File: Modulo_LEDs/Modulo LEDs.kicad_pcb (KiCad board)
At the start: 2 copper layers, 33 x 61.6 mm, 18 parts, among them J1 Conn_01x09_Female, J2 Conn_01x09_Male

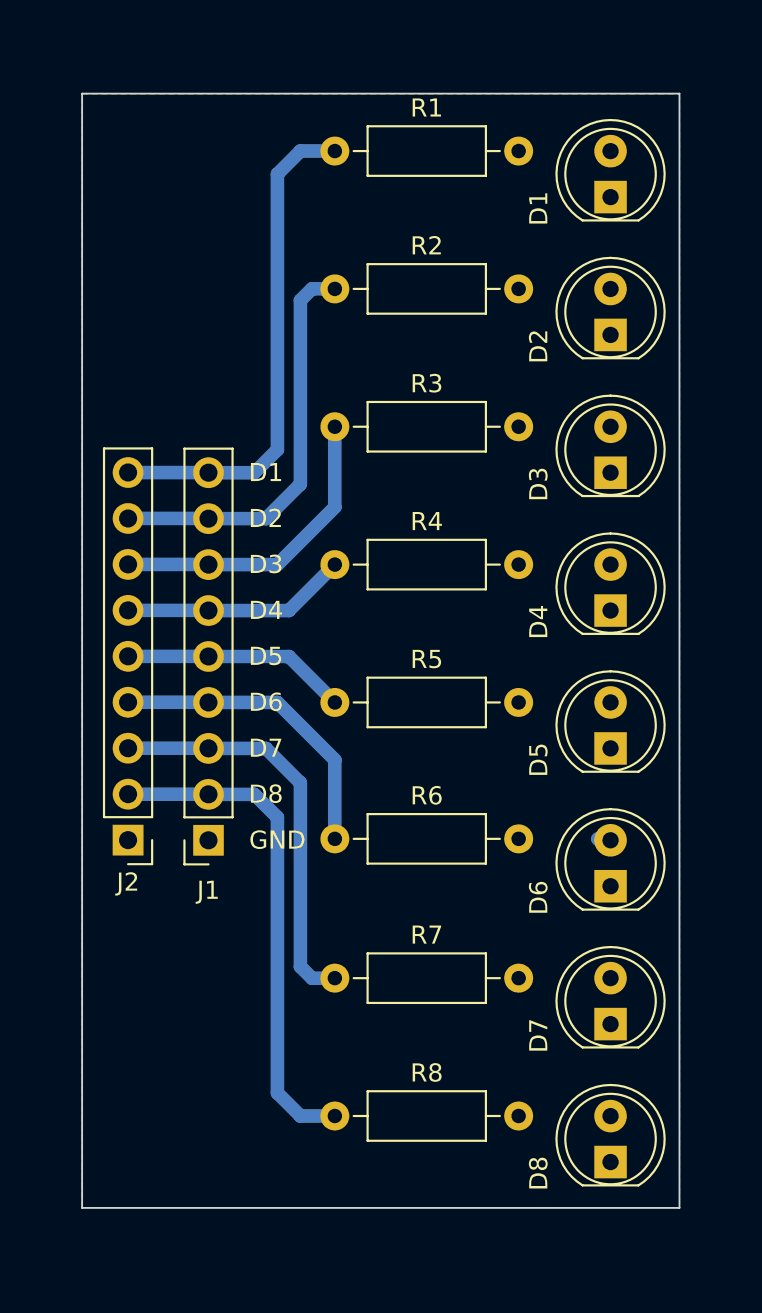
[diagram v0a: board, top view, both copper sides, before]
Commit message: Fixed PCb
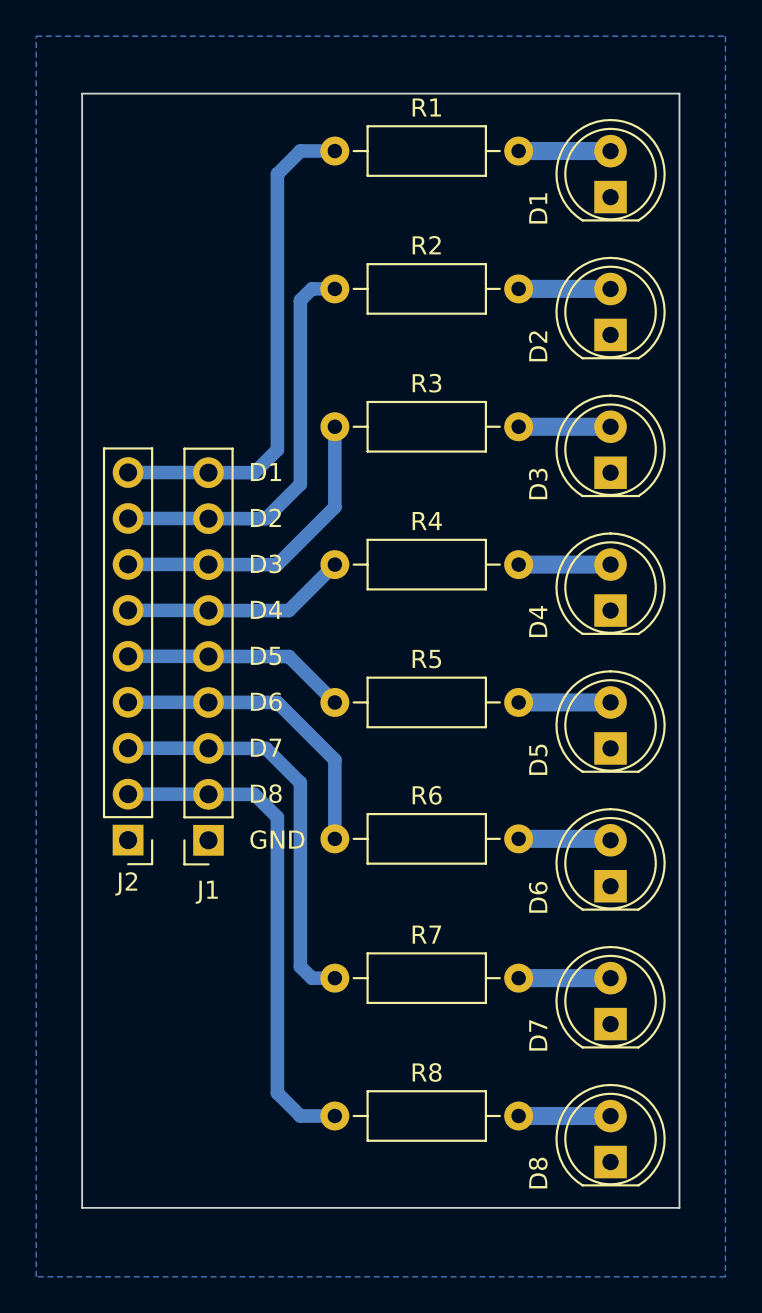
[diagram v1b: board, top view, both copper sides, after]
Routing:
- net Net-(D6-Pad2): track 0.11 -> 5.23 mm
- net Net-(D8-Pad2): track 0.00 -> 5.08 mm
- net Net-(D2-Pad2): track 0.00 -> 5.08 mm
- net Net-(D1-Pad2): track 0.00 -> 5.08 mm
- net Net-(D7-Pad2): track 0.00 -> 5.08 mm
- net Net-(D5-Pad2): track 0.00 -> 5.08 mm
- net Net-(D4-Pad2): track 0.00 -> 5.08 mm
- net Net-(D3-Pad2): track 0.00 -> 5.08 mm
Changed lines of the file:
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@@
     (style (thickness 0.15) (arrow_length 1.27) (text_position_mode 0) (extension_height 0.58642) (extension_offset 0.5) keep_text_aligned)
   )
+  (segment (start 86.36 81.28) (end 91.435 81.28) (width 1) (layer "B.Cu") (net 1))
+  (segment (start 91.435 81.28) (end 91.44 81.285) (width 1) (layer "B.Cu") (net 1))
+  (segment (start 86.36 88.9) (end 91.435 88.9) (width 1) (layer "B.Cu") (net 2))
+  (segment (start 91.435 88.9) (end 91.44 88.905) (width 1) (layer "B.Cu") (net 2))
+  (segment (start 86.36 96.52) (end 91.44 96.52) (width 1) (layer "B.Cu") (net 3))
+  (segment (start 86.36 104.14) (end 91.44 104.14) (width 1) (layer "B.Cu") (net 4))
+  (segment (start 86.36 111.76) (end 91.44 111.76) (width 1) (layer "B.Cu") (net 5))
+  (segment (start 91.36 119.3) (end 91.44 119.38) (width 1) (layer "B.Cu") (net 6))
   (segment (start 90.725 119.3) (end 90.805 119.38) (width 0.75) (layer "B.Cu") (net 6))
+  (segment (start 86.36 119.3) (end 91.36 119.3) (width 1) (layer "B.Cu") (net 6))
+  (segment (start 86.36 127) (end 91.44 127) (width 1) (layer "B.Cu") (net 7))
+  (segment (start 86.36 134.62) (end 91.435 134.62) (width 1) (layer "B.Cu") (net 8))
+  (segment (start 91.435 134.62) (end 91.44 134.625) (width 1) (layer "B.Cu") (net 8))
   (segment (start 71.755 116.84) (end 73.025 118.11) (width 0.75) (layer "B.Cu") (net 10))
   (segment (start 73.025 133.35) (end 74.295 134.62) (width 0.75) (layer "B.Cu") (net 10))
@@
     (polygon
       (pts
-        (xy 95.25 139.7)
-        (xy 62.23 139.7)
-        (xy 62.23 78.105)
-        (xy 95.25 78.105)
+        (xy 97.79 143.51)
+        (xy 59.69 143.51)
+        (xy 59.69 74.93)
+        (xy 97.79 74.93)
       )
     )
